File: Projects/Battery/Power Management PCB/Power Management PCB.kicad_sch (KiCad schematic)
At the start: 14 parts, among them U1 LM317_SOT-223

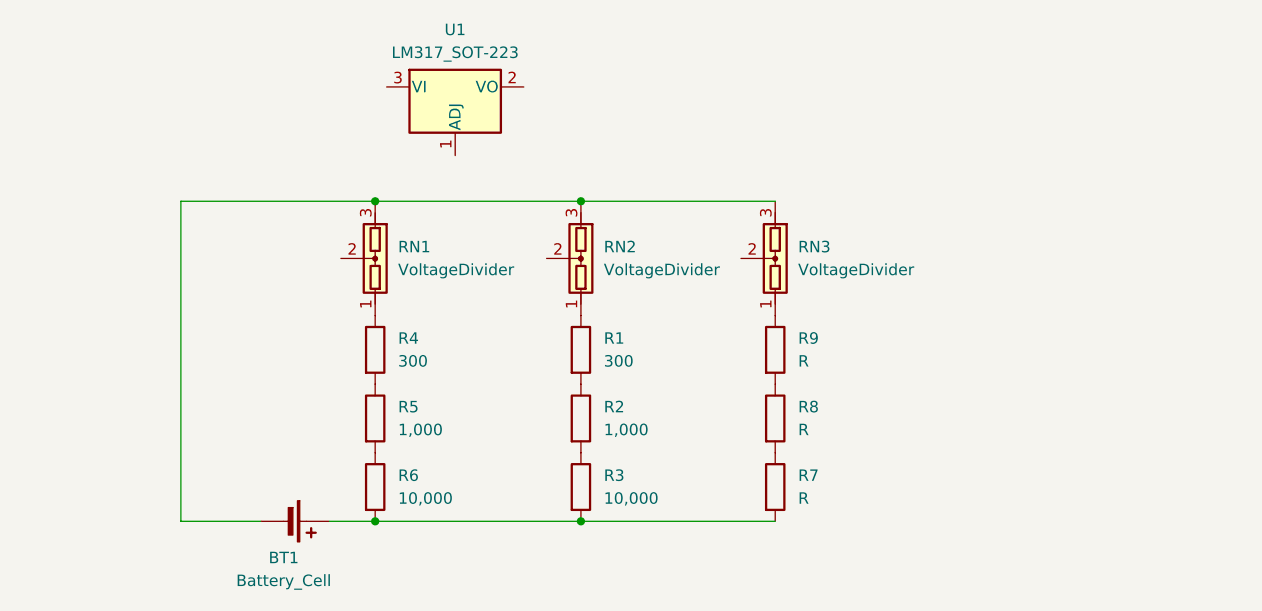
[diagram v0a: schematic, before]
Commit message: Update schematic and layout
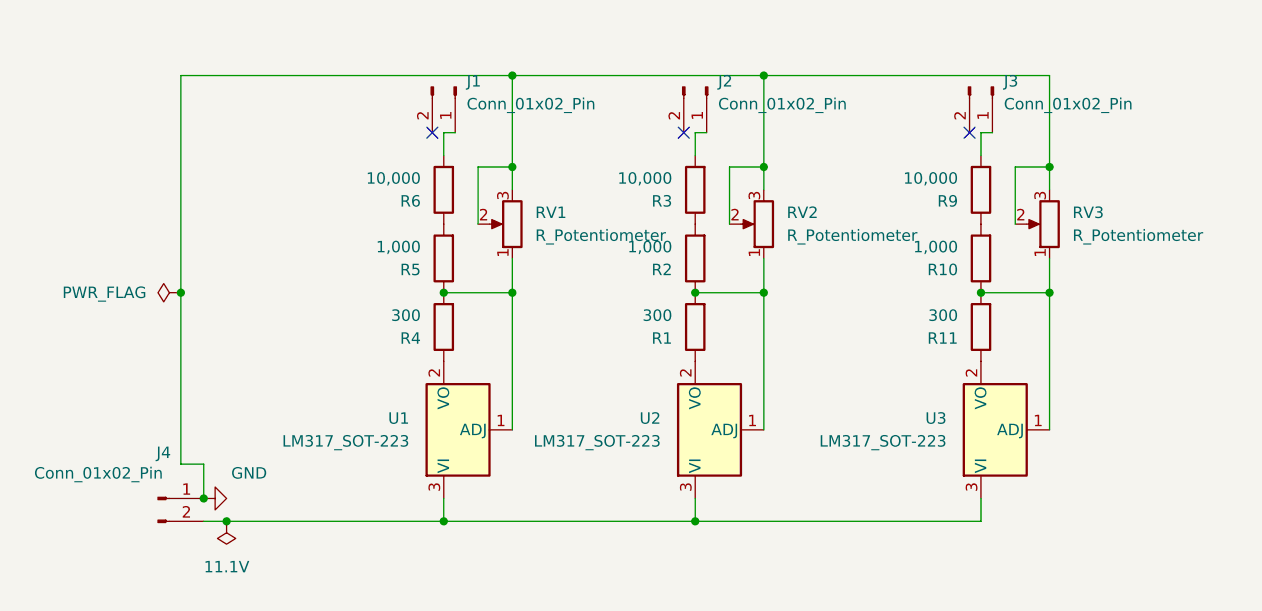
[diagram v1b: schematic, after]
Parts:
- removed BT1: Battery_Cell, symbol Device:Battery_Cell
- removed R7, R8: R, symbol Device:R
- removed RN1, RN2, RN3: VoltageDivider, symbol Device:VoltageDivider
- added J1, J2, J3, J4: Conn_01x02_Pin, Connector_PinHeader_1.27mm:PinHeader_1x02_P1.27mm_Vertical_SMD_Pin1Left, symbol Connector:Conn_01x02_Pin
- added R10: 1,000, Resistor_SMD:R_0201_0603Metric, symbol Device:R
- added R11: 300, Resistor_SMD:R_0201_0603Metric, symbol Device:R
- added RV1, RV2, RV3: R_Potentiometer, Potentiometer_SMD:Potentiometer_Bourns_3314J_Vertical, symbol Device:R_Potentiometer
- added U2, U3: LM317_SOT-223, Package_TO_SOT_SMD:SOT-223-3_TabPin2, symbol Regulator_Linear:LM317_SOT-223
- R1, R2, R3, R4, R5, R6: footprint (none) -> Resistor_SMD:R_0201_0603Metric
- R9: value R -> 10,000; footprint (none) -> Resistor_SMD:R_0201_0603Metric
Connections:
- net at R6.2: now also J1.1 (Pin_1); no longer R3.2
- net at R1.1: now also U2.2 (VO)
- net at R1.2, R2.1: now also RV2.1, U2.1 (ADJ)
- net at R9.1: now also R10.2
- net at R4.2, R5.1: now also U1.1 (ADJ), RV1.1
- net at U1.2 (VO): now also R4.1
- net at U1.3 (VI): now also J4.2 (Pin_2), U2.3 (VI), U3.3 (VI)
- net at R9.2: now also J3.1 (Pin_1)
- new net: J2.1 (Pin_1), R3.2
- new net: R10.1, R11.2, RV3.1, U3.1 (ADJ)
- new net: R11.1, U3.2 (VO)
- new net GND: J4.1 (Pin_1), RV1.2, RV1.3, RV2.2, RV2.3, RV3.2, RV3.3
- no-connect marks 0 -> 3
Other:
- moved on the sheet: R1, R2, R3, R4, R5, R6

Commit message: 9/22 pcb
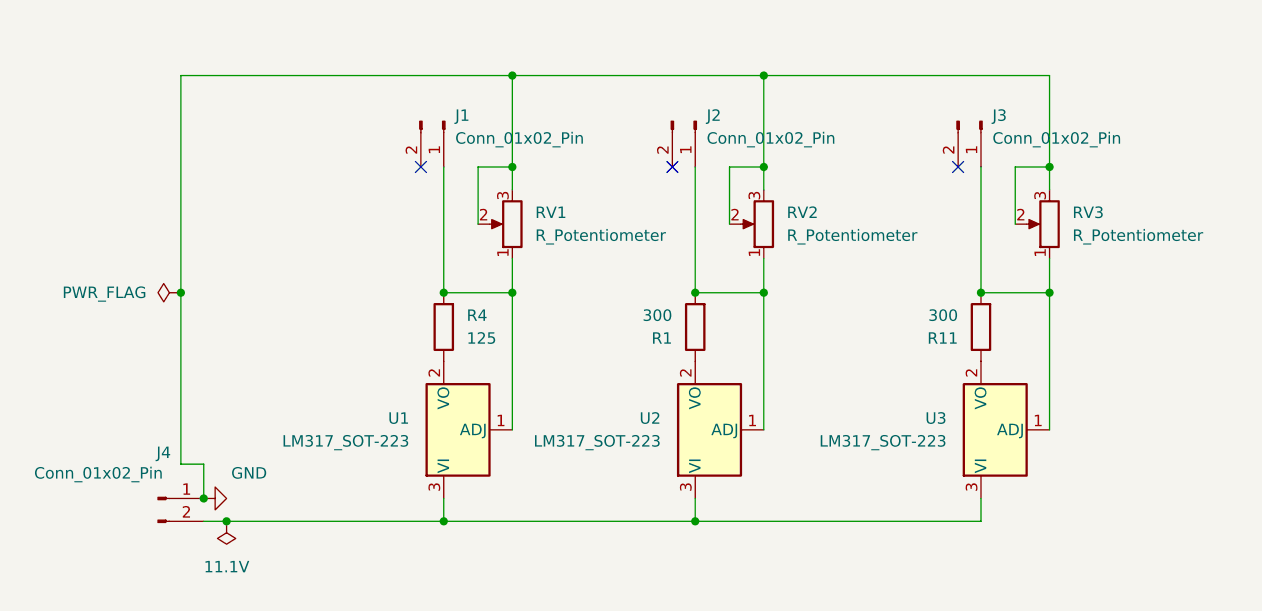
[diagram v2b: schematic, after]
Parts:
- removed R10, R2, R5: 1,000, Resistor_SMD:R_0201_0603Metric, symbol Device:R
- removed R3, R6, R9: 10,000, Resistor_SMD:R_0201_0603Metric, symbol Device:R
- R4: value 300 -> 125
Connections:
- net at J3.1 (Pin_1): now also R11.2, RV3.1, U3.1 (ADJ)
- net at J1.1 (Pin_1): now also R4.2, RV1.1, U1.1 (ADJ)
- net at R1.2, RV2.1, U2.1 (ADJ): now also J2.1 (Pin_1)
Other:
- moved on the sheet: J1, J2, J3
